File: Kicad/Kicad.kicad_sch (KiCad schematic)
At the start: 0 parts

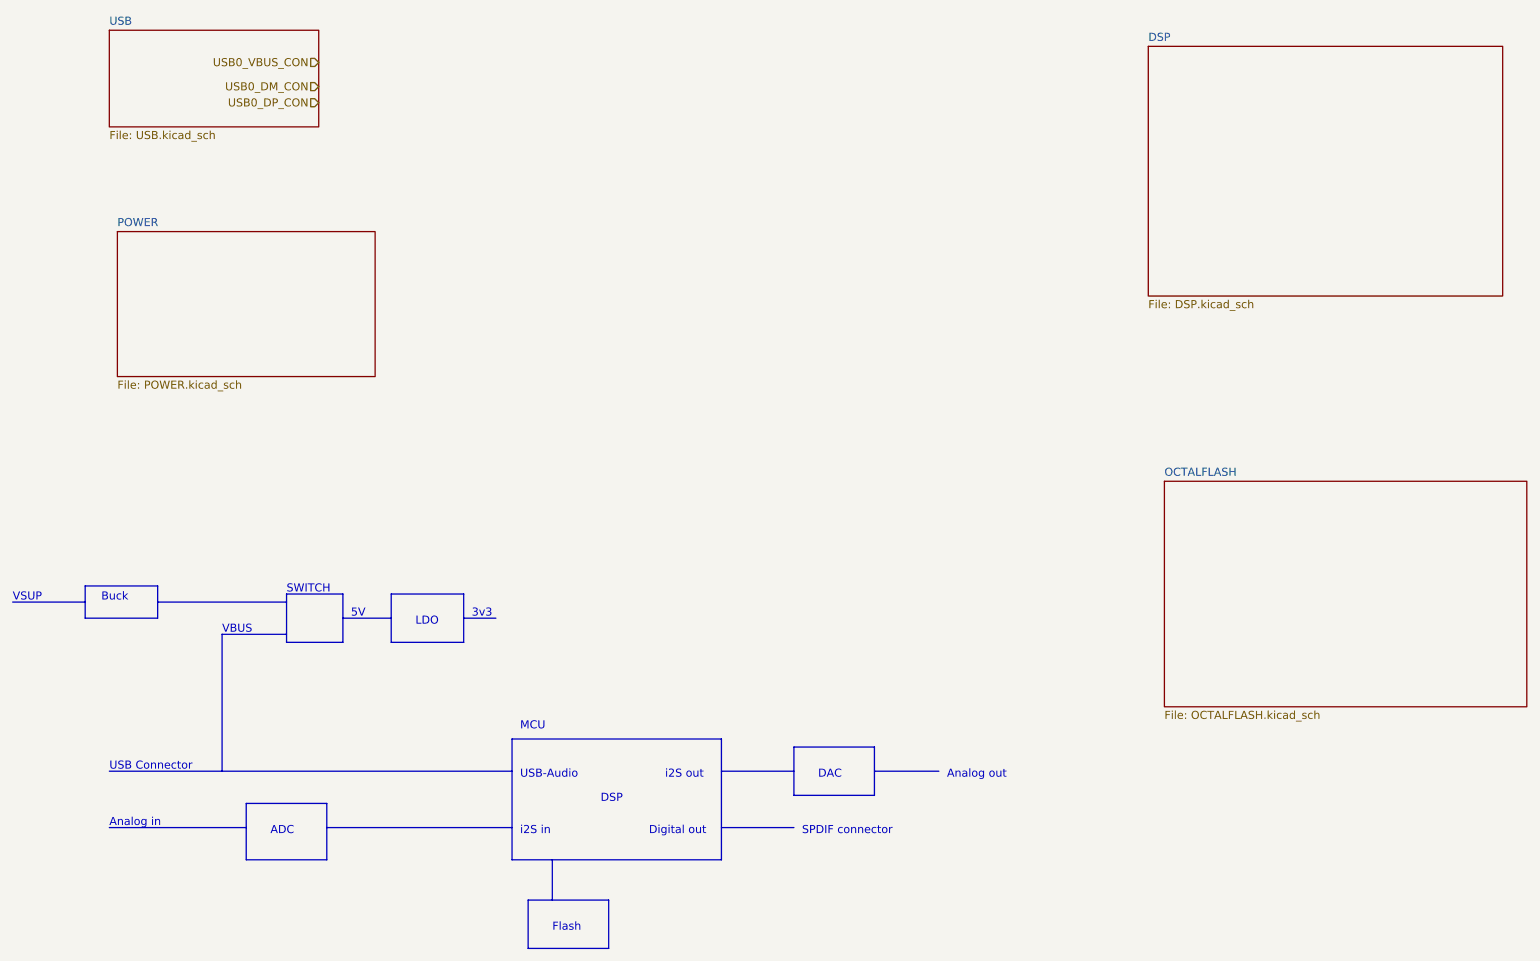
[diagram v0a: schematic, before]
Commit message: power section
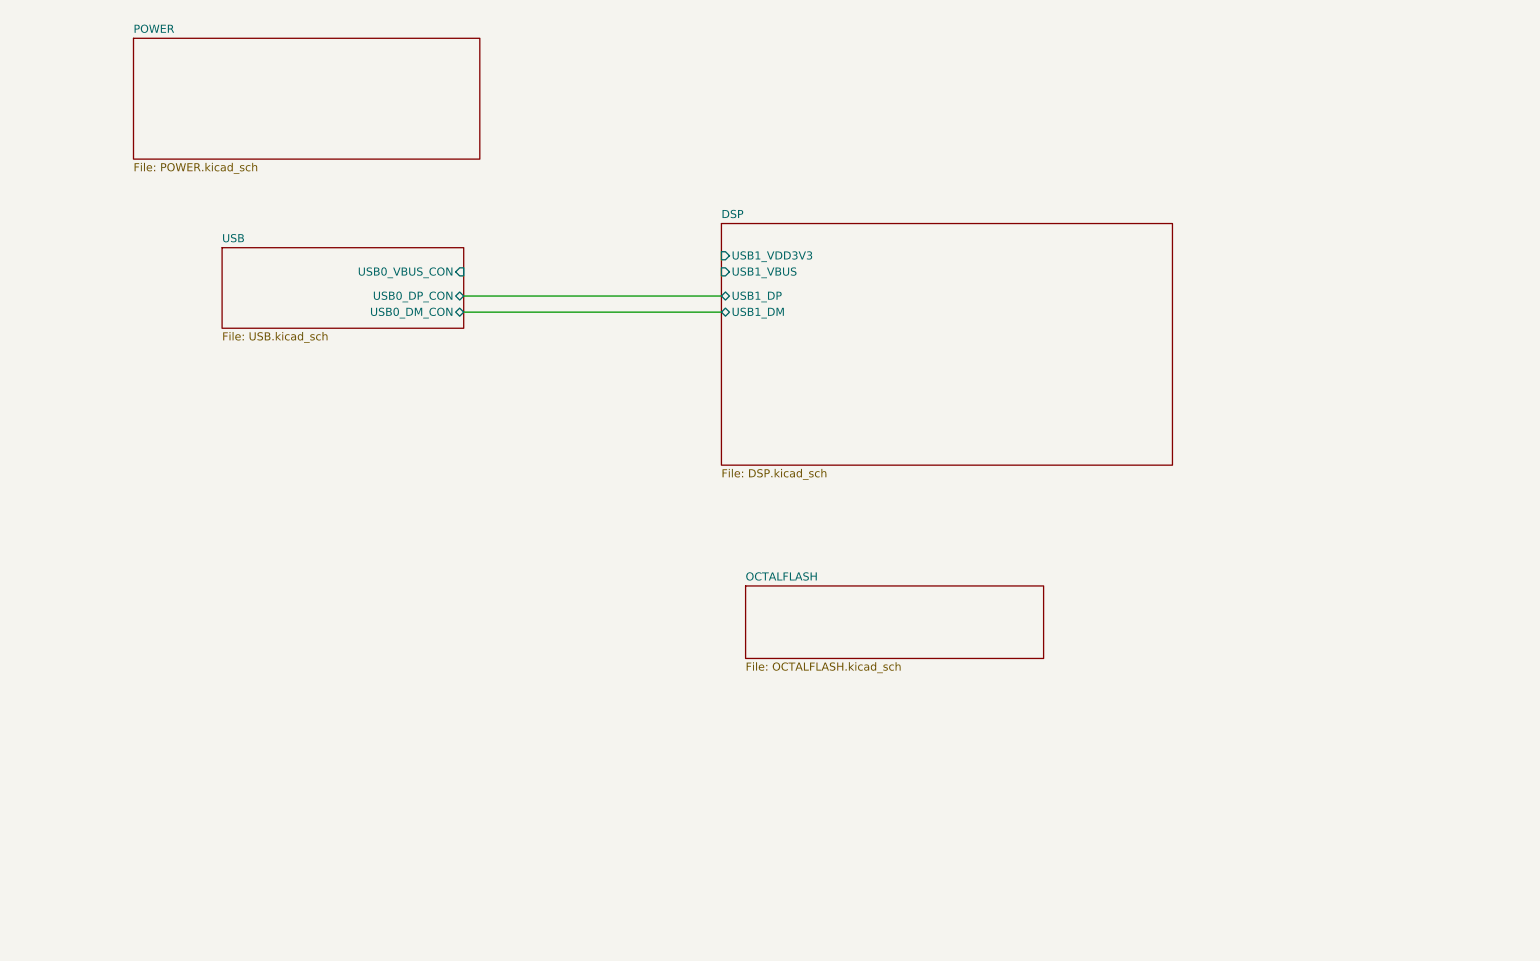
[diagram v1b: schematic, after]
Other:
- sheet DSP ports: added USB1_DM, USB1_DP, USB1_VBUS, USB1_VDD3V3; removed none
- sheet USB ports: added USB0_DM_CON, USB0_DP_CON, USB0_VBUS_CON; removed none
- note removed: "3v3"
- note removed: "5V"
- note removed: "ADC"
- note removed: "Analog in"
- note removed: "Analog out"
- note removed: "Buck"
- note removed: "DAC"
- note removed: "DSP"
- note removed: "Digital out"
- note removed: "Flash"
- note removed: "LDO"
- note removed: "MCU"
- note removed: "SPDIF connector"
- note removed: "SWITCH"
- note removed: "USB Connector"
- note removed: "USB-Audio"
- note removed: "VBUS"
- note removed: "VSUP"
- note removed: "i2S in"
- note removed: "i2S out"
